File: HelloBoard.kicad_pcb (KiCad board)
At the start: 2 copper layers, 96 x 71 mm, 43 parts, among them J1 USB_B_Micro, J2 Conn_01x04_Pin, J3 Conn_01x04_Pin, J4 Conn_02x08_Top_Bottom, J5 Conn_01x02, SW1 SW_Push, SW2 SW_Push, U1 STM32F103C8T6, U2 AMS1117-3.3, U3 TMP235A2DCKR, U4 ADXL343, Y1 16MHz

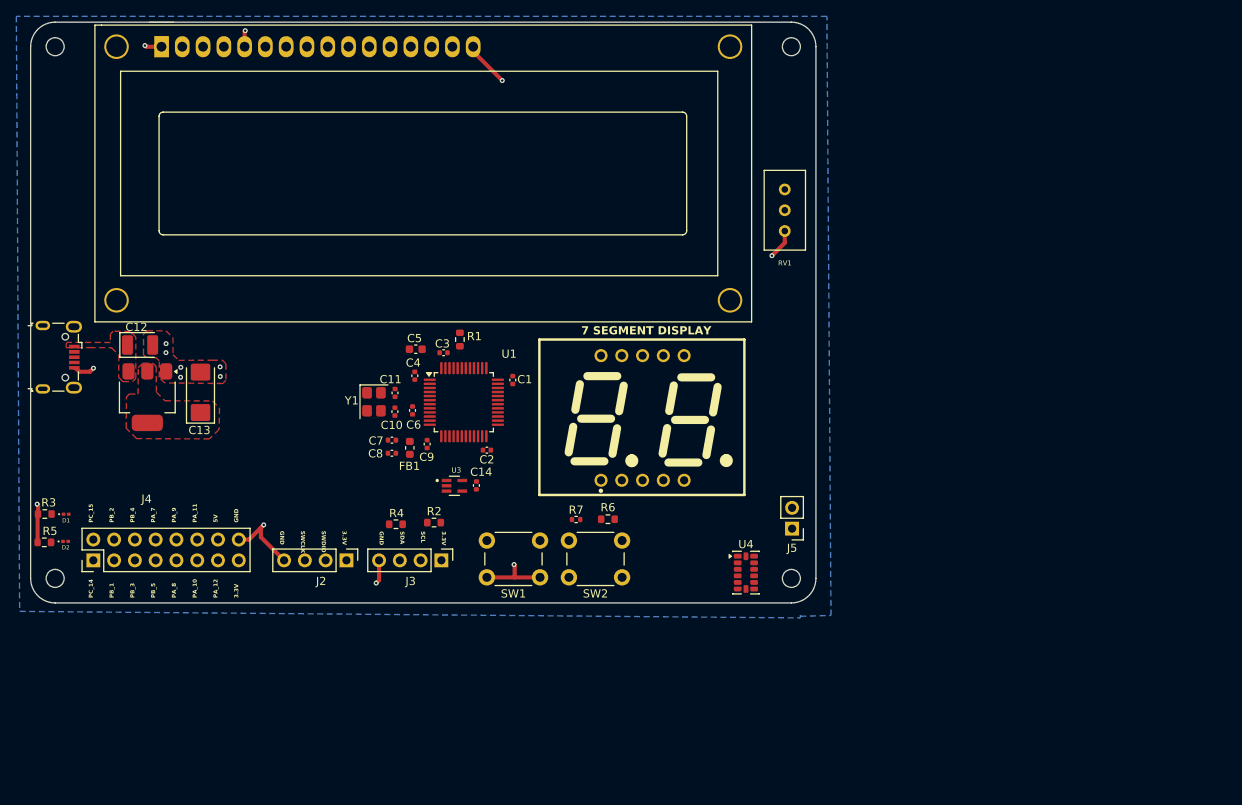
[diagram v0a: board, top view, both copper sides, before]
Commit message: حلتيته
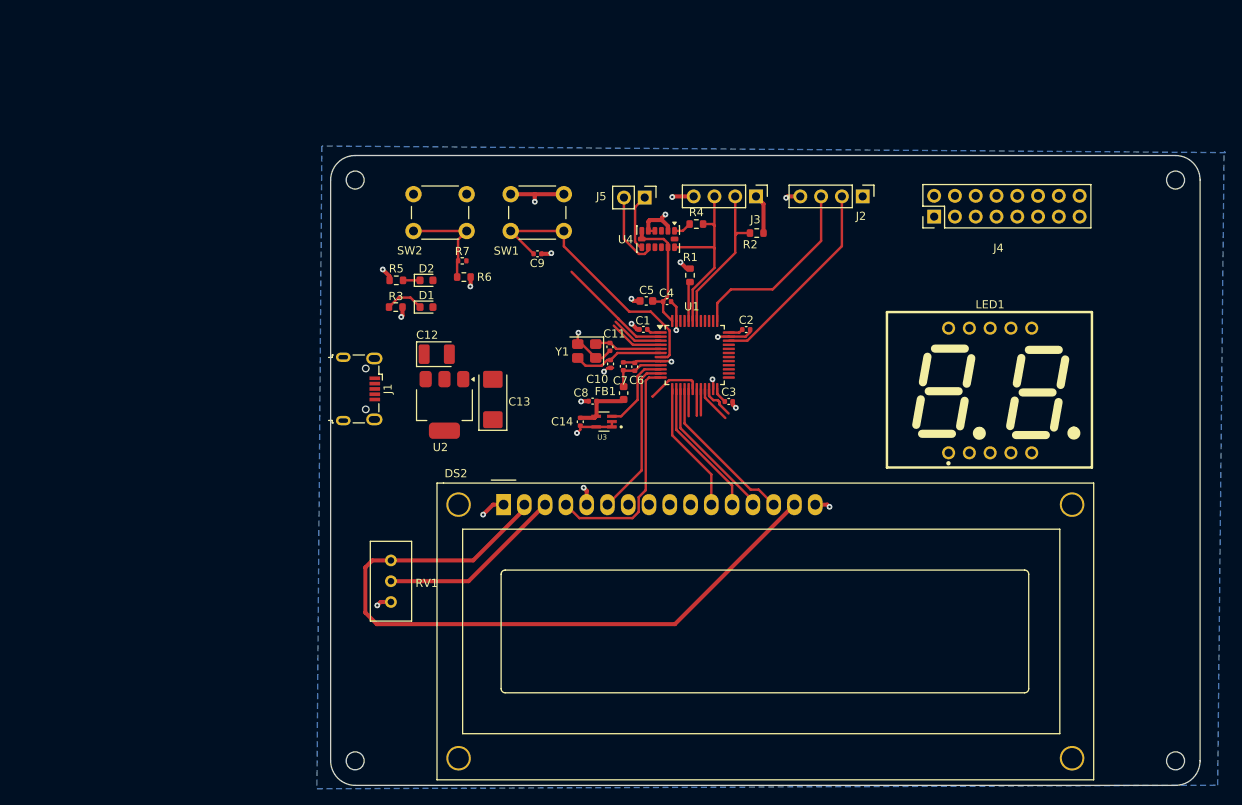
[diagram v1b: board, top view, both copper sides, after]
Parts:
- D1, D2: footprint LED_SMD:LED_0201_0603Metric -> LED_SMD:LED_0603_1608Metric
- moved H3 145.4 mm to (218.9, 41.0)
- moved J4 111.0 mm to (189.4, 45.5)
- moved H2 94.7 mm to (118.6, 112.0)
- moved J2 77.2 mm to (180.6, 43.0)
- moved DS2 69.9 mm to (136.7, 80.7)
- moved RV1 66.1 mm to (123.0, 87.5)
- moved J3 58.8 mm to (167.6, 43.0)
- moved H1 55.8 mm to (118.6, 41.0)
- moved D2 54.5 mm to (127.3, 53.2)
- moved R5 53.6 mm to (123.6, 53.2)
- moved SW2 53.3 mm to (125.7, 42.7), turned to 0 degrees
- moved R2 53.0 mm to (167.7, 47.5), turned to 180 degrees
- moved H4 52.0 mm to (218.9, 112.0)
- moved R4 51.9 mm to (160.3, 46.4), turned to 0 degrees
- moved D1 50.8 mm to (127.3, 56.5)
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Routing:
- net VBUS: track 0.00 -> 87.9 mm
- net +3.3V: track 0.00 -> 35.8 mm
- net /NRST: track 0.00 -> 33.7 mm
- net /LCD_RS: track 0.00 -> 28.7 mm
- net GND: track 40.8 -> 67.0 mm, vias 15 -> 24
- net /SWDIO: track 0.00 -> 24.7 mm
- net /SWCLK: track 0.00 -> 23.5 mm
- net /LCD_VO: track 0.00 -> 22.7 mm
- net /I2C_SDA: track 0.00 -> 22.7 mm
- net /LCD_E: track 0.00 -> 19.7 mm
- net /LCD_D7: track 0.00 -> 19.2 mm
- net /I2C_SCL: track 0.00 -> 19.0 mm
- net /LCD_D6: track 0.00 -> 17.8 mm
- net /LCD_D5: track 0.00 -> 17.0 mm
- net /LCD_D4: track 0.00 -> 16.1 mm
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- removed copper zone on F.Cu, net +3.3V
- removed copper zone on F.Cu, net GND
- removed copper zone on F.Cu, net VBUS
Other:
- board size 96 x 71 mm -> 106.3 x 77 mm
- board text removed: "3.3V"
- board text removed: "5V"
- board text removed: "7 SEGMENT DISPLAY"
- board text removed: "GND"
- board text removed: "PA_10"
- board text removed: "PA_11"
- board text removed: "PA_12"
- board text removed: "PA_7"
- board text removed: "PA_8"
- board text removed: "PA_9"
- board text removed: "PB_1"
- board text removed: "PB_2"
- board text removed: "PB_3"
- board text removed: "PB_4"
- board text removed: "PB_5"
- board text removed: "PC_14"
- board text removed: "PC_15"
- board text removed: "SCL"
- board text removed: "SDA"
- board text removed: "SWCLK"
- board text removed: "SWDIO"
